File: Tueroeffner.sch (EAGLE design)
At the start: 41 parts, among them IC1 NCP1117ST33T3G, IC3 M25PE20, K2 EC2-12TNU, Q1 2N7002CK, Q2 2N7002CK

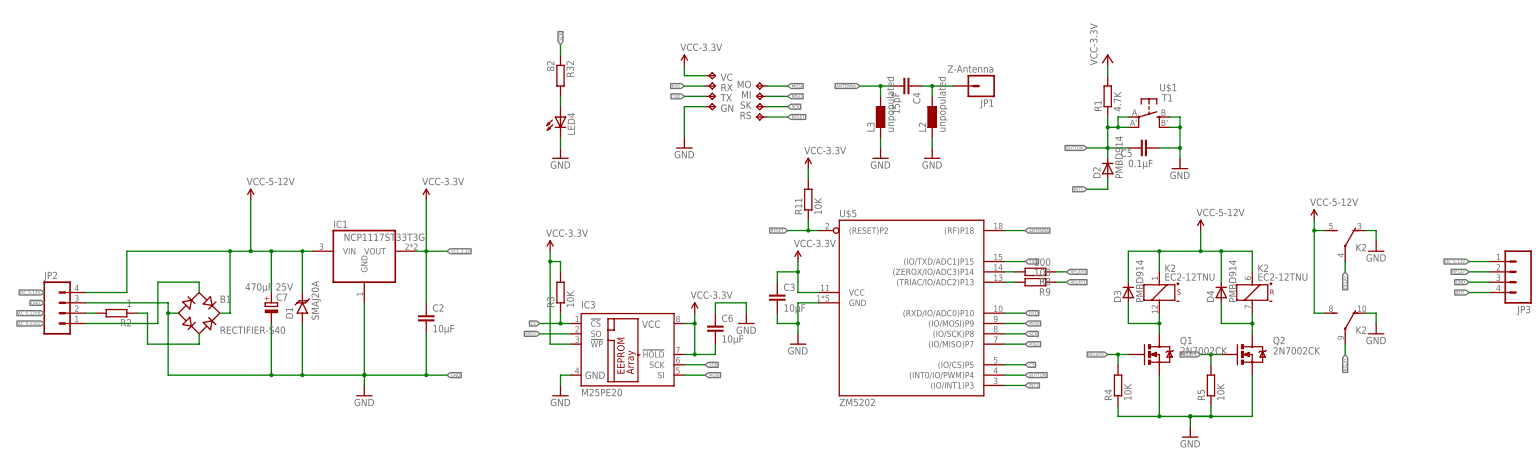
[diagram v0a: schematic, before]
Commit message: Final RC
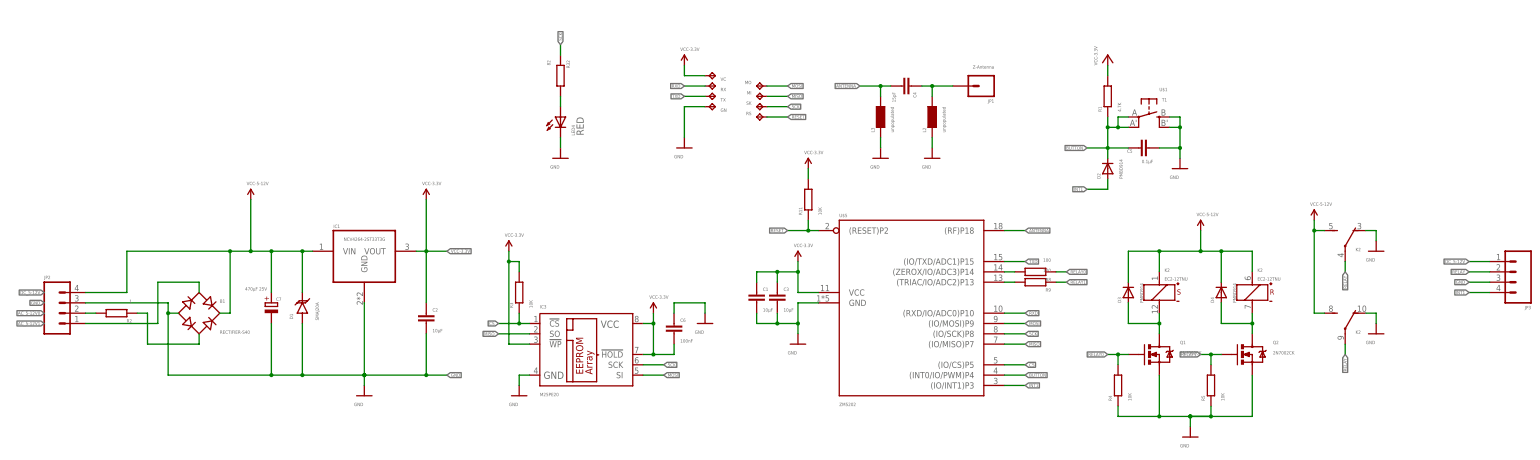
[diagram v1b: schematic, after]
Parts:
- added C1: 10µF, eagle-ltspice:CC2012
- C6: value 10µF -> 100nF
- IC1: value NCP1117ST33T3G -> NCV4264-2ST33T3G; device burr-brown:REG1117 -> burr-brown:REG1118
- LED4: value (none) -> RED
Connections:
- net GND: now also C1.2
- net VCC-3.3V: now also C1.1
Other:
- moved on the sheet: C6, IC1, IC3, R3
